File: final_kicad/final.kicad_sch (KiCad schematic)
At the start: 43 parts, among them J1 Signal, J11 MCU_power_pin, J2 Battery, J3 Power, J4 SDA, J5 PIN1, J6 PIN2, J7 SCL, J8 PIN3, J9 PIN4, M1 Motor_DC, M2 Motor_DC, Q1 NPN, Q2 NPN, SW1 SW_SPST, SW2 SW_Push, SW3 SW_Push, SW5 SW_SPST, U1 MPU-6050, U2 MPU-6050

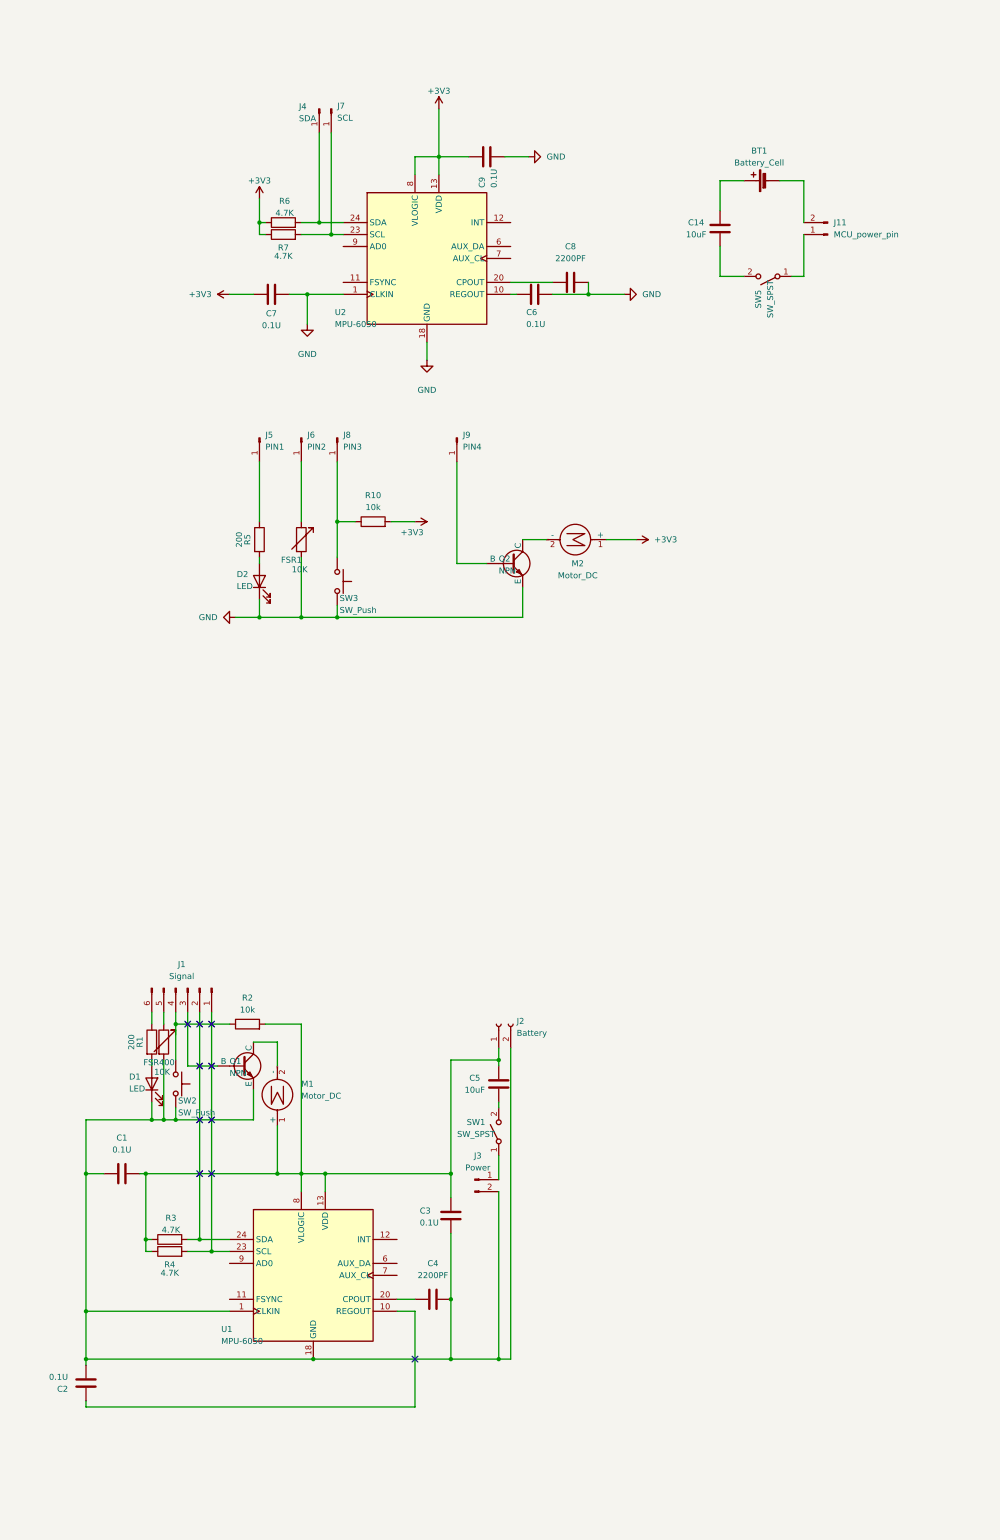
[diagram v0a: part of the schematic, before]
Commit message: 1
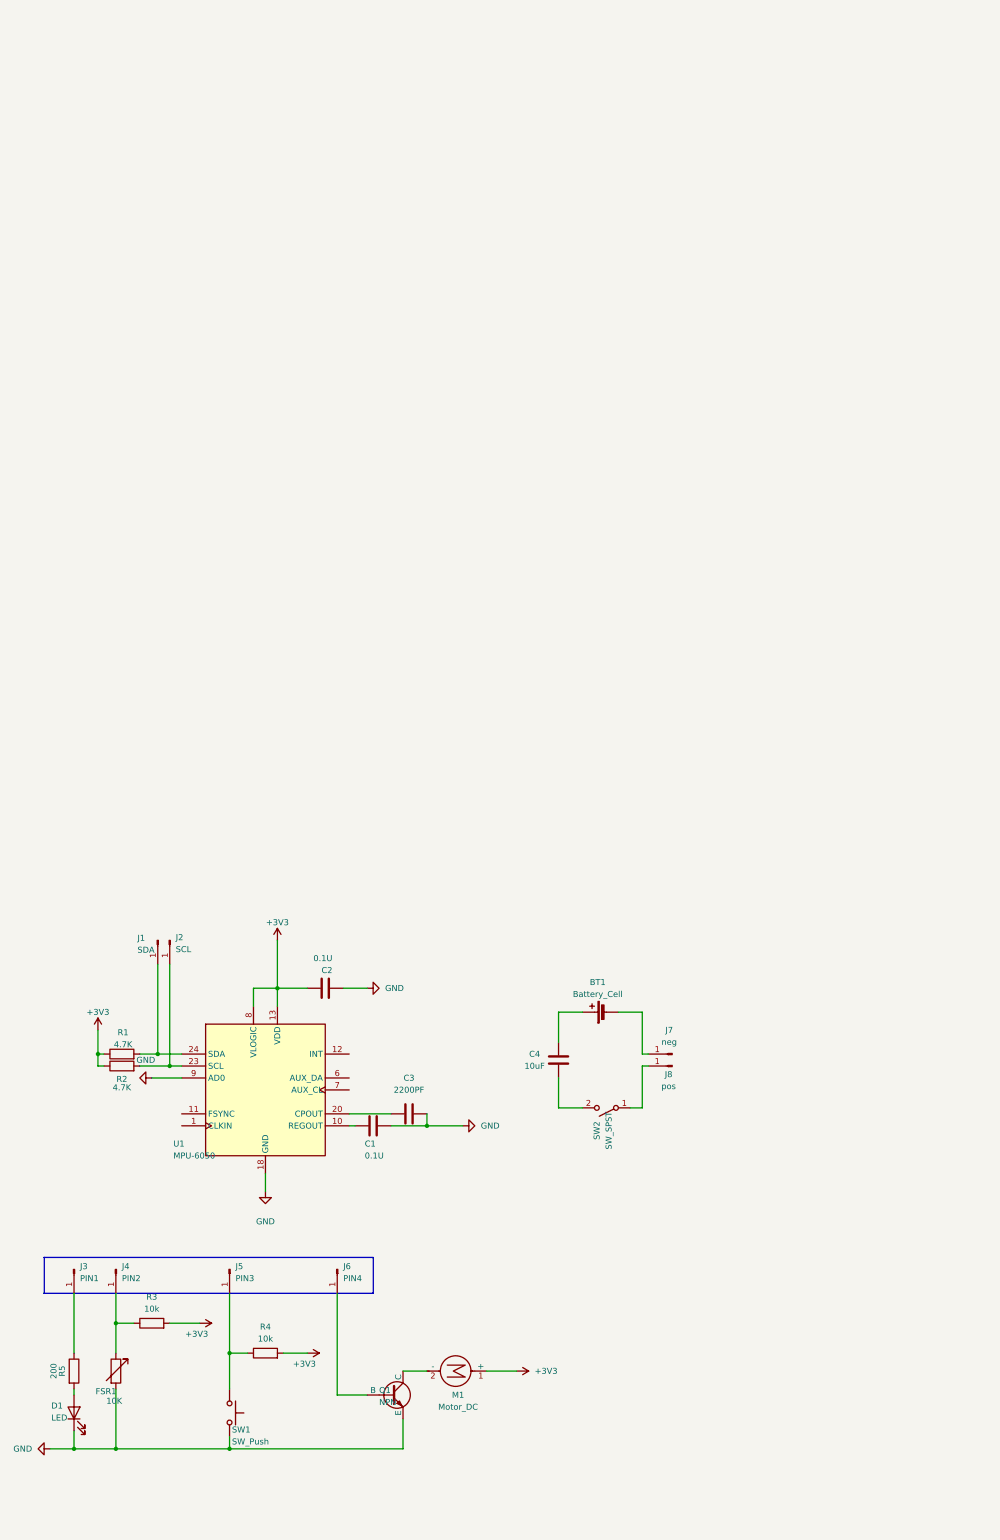
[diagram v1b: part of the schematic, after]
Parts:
- removed C1, C2, C3, C7: 0.1U, Capacitor_SMD:C_0603_1608Metric, symbol Device:C
- removed C4: 2200PF, Capacitor_SMD:C_0603_1608Metric, symbol Device:C
- removed C5: 10uF, Capacitor_SMD:C_0603_1608Metric, symbol Device:C
- removed D1: LED, LED_THT:LED_D3.0mm, symbol Device:LED
- removed FSR400: 10K, Connector_PinHeader_1.00mm:PinHeader_1x02_P1.00mm_Vertical, symbol Device:R_Variable
- removed J1: Signal, Connector_PinHeader_1.00mm:PinHeader_1x06_P1.00mm_Vertical, symbol Connector:Conn_01x06_Pin
- removed J11: MCU_power_pin, Connector_PinHeader_1.00mm:PinHeader_1x02_P1.00mm_Vertical, symbol Connector:Conn_01x02_Pin
- removed J2: Battery, Connector_JST:JST_PH_B2B-PH-K_1x02_P2.00mm_Vertical, symbol Connector:Conn_01x02_Socket
- removed J3: Power, Connector_PinHeader_1.00mm:PinHeader_1x02_P1.00mm_Vertical, symbol Connector:Conn_01x02_Pin
- removed M1: Motor_DC, Connector_PinHeader_1.00mm:PinHeader_1x02_P1.00mm_Vertical, symbol Motor:Motor_DC
- removed Q1: NPN, Crystal:Resonator-3Pin_W6.0mm_H3.0mm, symbol Simulation_SPICE:NPN
- removed R1: 200, Resistor_SMD:R_0603_1608Metric, symbol Device:R
- removed R2: 10k, Resistor_SMD:R_0603_1608Metric, symbol Device:R
- removed R4: 4.7K, Resistor_SMD:R_0603_1608Metric, symbol Device:R
- removed SW1: SW_SPST, Button_Switch_THT:SW_DIP_SPSTx01_Slide_6.7x4.1mm_W7.62mm_P2.54mm_LowProfile, symbol Switch:SW_SPST
- removed SW2: SW_Push, Button_Switch_THT:SW_PUSH_6mm, symbol Switch:SW_Push
- removed U1: MPU-6050, Sensor_Motion:InvenSense_QFN-24_4x4mm_P0.5mm, symbol Sensor_Motion:MPU-6050
- added J7: neg, Connector_PinHeader_1.00mm:PinHeader_1x01_P1.00mm_Vertical, symbol Connector:Conn_01x01_Pin
- added J8: pos, Connector_PinHeader_1.00mm:PinHeader_1x01_P1.00mm_Vertical, symbol Connector:Conn_01x01_Pin
- J1: renamed from J4; footprint Connector_Wire:SolderWire-0.1sqmm_1x01_D0.4mm_OD1mm -> Connector_PinHeader_1.00mm:PinHeader_1x01_P1.00mm_Vertical
- J2: renamed from J7; footprint Connector_Wire:SolderWire-0.1sqmm_1x01_D0.4mm_OD1mm -> Connector_PinHeader_1.00mm:PinHeader_1x01_P1.00mm_Vertical
- J3: renamed from J5; footprint Connector_Wire:SolderWire-0.1sqmm_1x01_D0.4mm_OD1mm -> Connector_PinHeader_1.00mm:PinHeader_1x01_P1.00mm_Vertical
- J4: renamed from J6; footprint Connector_Wire:SolderWire-0.1sqmm_1x01_D0.4mm_OD1mm -> Connector_PinHeader_1.00mm:PinHeader_1x01_P1.00mm_Vertical
- J5: renamed from J8; footprint Connector_Wire:SolderWire-0.1sqmm_1x01_D0.4mm_OD1mm -> Connector_PinHeader_1.00mm:PinHeader_1x01_P1.00mm_Vertical
- J6: renamed from J9; footprint Connector_Wire:SolderWire-0.1sqmm_1x01_D0.4mm_OD1mm -> Connector_PinHeader_1.00mm:PinHeader_1x01_P1.00mm_Vertical
- R3: value 4.7K -> 10k
- renumbered C6 to C1, C9 to C2, C8 to C3, C14 to C4, D2 to D1, M2 to M1, Q2 to Q1, R6 to R1, R7 to R2, R10 to R4, SW3 to SW1, SW5 to SW2, U2 to U1
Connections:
- net +3V3: now also R3.2
- net GND: now also U1.9 (AD0); no longer U1.1 (CLKIN)
- net at SW2.1 (A): now also J8.1 (Pin_1)
- net at FSR1.1, J4.1 (Pin_1): now also R3.1
- net at BT1.2 (-): now also J7.1 (Pin_1)
- no-connect marks 13 -> 3
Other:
- moved on the sheet: BT1, C1, C2, C3, C4, D1, FSR1, J1, J2, J3, J4, J5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
